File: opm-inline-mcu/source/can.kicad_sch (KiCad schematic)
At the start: 34 parts, among them IC2 RP2040, IC3 RP2040, IC4 RP2040, IC5 MIC5219-3.3YM5-TR, IC6 MIC5219-5.0YM5-TR, IC7 TJA1051TK{slash}3, Q8 CSTCE8M00G55-R0

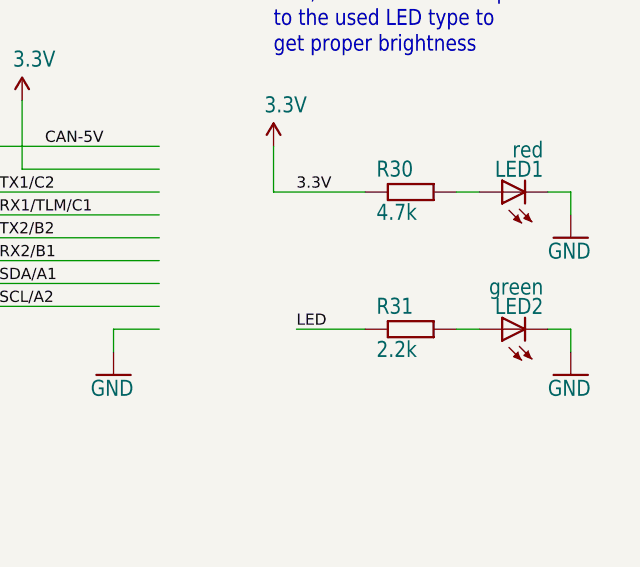
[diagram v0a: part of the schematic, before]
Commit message: update for can
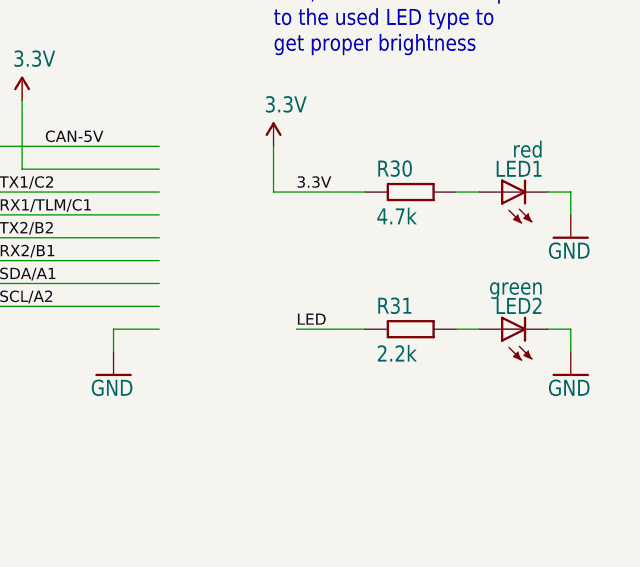
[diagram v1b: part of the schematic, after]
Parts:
- C28: footprint Resistor_SMD:R_0603_1608Metric -> Capacitor_SMD:C_0603_1608Metric
- C29, C30, C35: footprint uc4h node v2100:C0603K -> Capacitor_SMD:C_0603_1608Metric
- F1: footprint uc4h node v2100:FUSE-0805 -> uc4h node v2100.pretty:FUSE-0805
- IC5, IC6: footprint uc4h node v2100:SOT23-5 -> uc4h node v2100.pretty:SOT23-5
- IC7: footprint uc4h node v2100:HVSON8 -> uc4h node v2100.pretty:HVSON8
- JP2: footprint uc4h node v2100:1X01 -> uc4h node v2100.pretty:1X01
- JP3: footprint uc4h node v2100:1X02 -> uc4h node v2100.pretty:1X02
- JP4, JP5: footprint uc4h node v2100:SM04B-GHS-TB -> uc4h node v2100.pretty:SM04B-GHS-TB
- LED1, LED2: footprint uc4h node v2100:CHIPLED_0603 -> uc4h node v2100.pretty:CHIPLED_0603
- Q8: footprint uc4h node v2100:RESONATOR-SMD -> uc4h node v2100.pretty:RESONATOR-SMD
- R23, R29, R30, R31: footprint uc4h node v2100:R0603 -> Resistor_SMD:R_0603_1608Metric
- SJ1: footprint uc4h node v2100:SJ_2S-NO -> uc4h node v2100.pretty:SJ_2S-NO
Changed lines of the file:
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@@
       (effects (font (size 1.778 1.5113)) (justify left bottom))
     )
-    (property "Footprint" "uc4h node v2100:SJ_2S-NO" (id 2) (at 43.18 101.6 0)
+    (property "Footprint" "uc4h node v2100.pretty:SJ_2S-NO" (id 2) (at 43.18 101.6 0)
       (effects (font (size 1.27 1.27)) hide)
     )
@@
       (effects (font (size 1.778 1.5113)) (justify left bottom))
     )
-    (property "Footprint" "uc4h node v2100:1X02" (id 2) (at 182.88 124.46 0)
+    (property "Footprint" "uc4h node v2100.pretty:1X02" (id 2) (at 182.88 124.46 0)
       (effects (font (size 1.27 1.27)) hide)
     )
@@
       (effects (font (size 1.778 1.5113)) (justify right top))
     )
-    (property "Footprint" "uc4h node v2100:SM04B-GHS-TB" (id 2) (at 246.38 53.34 0)
+    (property "Footprint" "uc4h node v2100.pretty:SM04B-GHS-TB" (id 2) (at 246.38 53.34 0)
       (effects (font (size 1.27 1.27)) hide)
     )
@@
       (effects (font (size 1.778 1.5113)) (justify left bottom))
     )
-    (property "Footprint" "uc4h node v2100:C0603K" (id 2) (at 48.26 76.2 0)
+    (property "Footprint" "Capacitor_SMD:C_0603_1608Metric" (id 2) (at 48.26 76.2 0)
       (effects (font (size 1.27 1.27)) hide)
     )
@@
       (effects (font (size 1.778 1.5113)) (justify left bottom))
     )
-    (property "Footprint" "uc4h node v2100:CHIPLED_0603" (id 2) (at 259.08 137.16 0)
+    (property "Footprint" "uc4h node v2100.pretty:CHIPLED_0603" (id 2) (at 259.08 137.16 0)
       (effects (font (size 1.27 1.27)) hide)
     )
@@
       (effects (font (size 1.778 1.5113)) (justify left bottom))
     )
-    (property "Footprint" "uc4h node v2100:SOT23-5" (id 2) (at 104.14 170.18 0)
+    (property "Footprint" "uc4h node v2100.pretty:SOT23-5" (id 2) (at 104.14 170.18 0)
       (effects (font (size 1.27 1.27)) hide)
     )
@@
       (effects (font (size 1.778 1.5113)) (justify left bottom))
     )
-    (property "Footprint" "uc4h node v2100:R0603" (id 2) (at 205.74 93.98 0)
+    (property "Footprint" "Resistor_SMD:R_0603_1608Metric" (id 2) (at 205.74 93.98 0)
       (effects (font (size 1.27 1.27)) hide)
     )
@@
       (effects (font (size 1.778 1.5113)) (justify left bottom))
     )
-    (property "Footprint" "uc4h node v2100:RESONATOR-SMD" (id 2) (at 48.26 33.02 0)
+    (property "Footprint" "uc4h node v2100.pretty:RESONATOR-SMD" (id 2) (at 48.26 33.02 0)
       (effects (font (size 1.27 1.27)) hide)
     )
@@
       (effects (font (size 1.778 1.5113)) (justify left bottom))
     )
-    (property "Footprint" "uc4h node v2100:C0603K" (id 2) (at 40.64 111.76 0)
+    (property "Footprint" "Capacitor_SMD:C_0603_1608Metric" (id 2) (at 40.64 111.76 0)
       (effects (font (size 1.27 1.27)) hide)
     )
@@
       (effects (font (size 1.778 1.5113)) (justify left bottom))
     )
-    (property "Footprint" "uc4h node v2100:FUSE-0805" (id 2) (at 195.58 53.34 0)
+    (property "Footprint" "uc4h node v2100.pretty:FUSE-0805" (id 2) (at 195.58 53.34 0)
       (effects (font (size 1.27 1.27)) hide)
     )
@@
       (effects (font (size 1.778 1.5113)) (justify left bottom))
     )
-    (property "Footprint" "uc4h node v2100:CHIPLED_0603" (id 2) (at 259.08 152.4 0)
+    (property "Footprint" "uc4h node v2100.pretty:CHIPLED_0603" (id 2) (at 259.08 152.4 0)
       (effects (font (size 1.27 1.27)) hide)
     )
@@
       (effects (font (size 1.778 1.5113)) (justify left bottom))
     )
-    (property "Footprint" "uc4h node v2100:SOT23-5" (id 2) (at 109.22 134.62 0)
+    (property "Footprint" "uc4h node v2100.pretty:SOT23-5" (id 2) (at 109.22 134.62 0)
       (effects (font (size 1.27 1.27)) hide)
     )
@@
       (effects (font (size 1.778 1.5113)) (justify left bottom))
     )
-    (property "Footprint" "uc4h node v2100:C0603K" (id 2) (at 154.94 83.82 0)
+    (property "Footprint" "Capacitor_SMD:C_0603_1608Metric" (id 2) (at 154.94 83.82 0)
       (effects (font (size 1.27 1.27)) hide)
     )
@@
       (effects (font (size 1.778 1.5113)) (justify left bottom))
     )
-    (property "Footprint" "Resistor_SMD:R_0603_1608Metric" (id 2) (at 40.64 76.2 0)
+    (property "Footprint" "Capacitor_SMD:C_0603_1608Metric" (id 2) (at 40.64 76.2 0)
       (effects (font (size 1.27 1.27)) hide)
     )
@@
       (effects (font (size 1.778 1.5113)) (justify right top))
     )
-    (property "Footprint" "uc4h node v2100:SM04B-GHS-TB" (id 2) (at 246.38 73.66 0)
+    (property "Footprint" "uc4h node v2100.pretty:SM04B-GHS-TB" (id 2) (at 246.38 73.66 0)
       (effects (font (size 1.27 1.27)) hide)
     )
@@
       (effects (font (size 1.778 1.5113)) (justify left bottom))
     )
-    (property "Footprint" "uc4h node v2100:R0603" (id 2) (at 50.8 119.38 0)
+    (property "Footprint" "Resistor_SMD:R_0603_1608Metric" (id 2) (at 50.8 119.38 0)
       (effects (font (size 1.27 1.27)) hide)
     )
@@
       (effects (font (size 1.778 1.5113)) (justify left bottom))
     )
-    (property "Footprint" "uc4h node v2100:HVSON8" (id 2) (at 180.34 81.28 0)
+    (property "Footprint" "uc4h node v2100.pretty:HVSON8" (id 2) (at 180.34 81.28 0)
       (effects (font (size 1.27 1.27)) hide)
     )
@@
       (effects (font (size 1.778 1.5113)) (justify left bottom))
     )
-    (property "Value" "4.7k" (id 1) (at 245.11 140.462 0)
-      (effects (font (size 1.778 1.5113)) (justify left bottom))
-    )
-    (property "Footprint" "uc4h node v2100:R0603" (id 2) (at 248.92 137.16 0)
+    (property "Value" "4.7k" (id 1) (at 245.11 140.97 0)
+      (effects (font (size 1.778 1.5113)) (justify left bottom))
+    )
+    (property "Footprint" "Resistor_SMD:R_0603_1608Metric" (id 2) (at 248.92 137.16 0)
       (effects (font (size 1.27 1.27)) hide)
     )
@@
       (effects (font (size 1.778 1.5113)) (justify left bottom))
     )
-    (property "Value" "2.2k" (id 1) (at 245.11 155.702 0)
-      (effects (font (size 1.778 1.5113)) (justify left bottom))
-    )
-    (property "Footprint" "uc4h node v2100:R0603" (id 2) (at 248.92 152.4 0)
+    (property "Value" "2.2k" (id 1) (at 245.11 156.21 0)
+      (effects (font (size 1.778 1.5113)) (justify left bottom))
+    )
+    (property "Footprint" "Resistor_SMD:R_0603_1608Metric" (id 2) (at 248.92 152.4 0)
       (effects (font (size 1.27 1.27)) hide)
     )
@@
       (effects (font (size 1.778 1.5113)) (justify left bottom))
     )
-    (property "Footprint" "uc4h node v2100:1X01" (id 2) (at 182.88 114.3 0)
-      (effects (font (size 1.27 1.27)) hide)
-    )
+    (property "Footprint" "uc4h node v2100.pretty:1X01" (id 2) (at 182.88 114.3 0)
+      (effects (font (size 1.27 1.27)) hide)
+    )
